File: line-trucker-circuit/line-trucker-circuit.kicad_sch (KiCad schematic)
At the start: 13 parts, among them Q1 Q_Photo_NPN, Q2 Q_Photo_NPN, Q3 Q_Photo_NPN

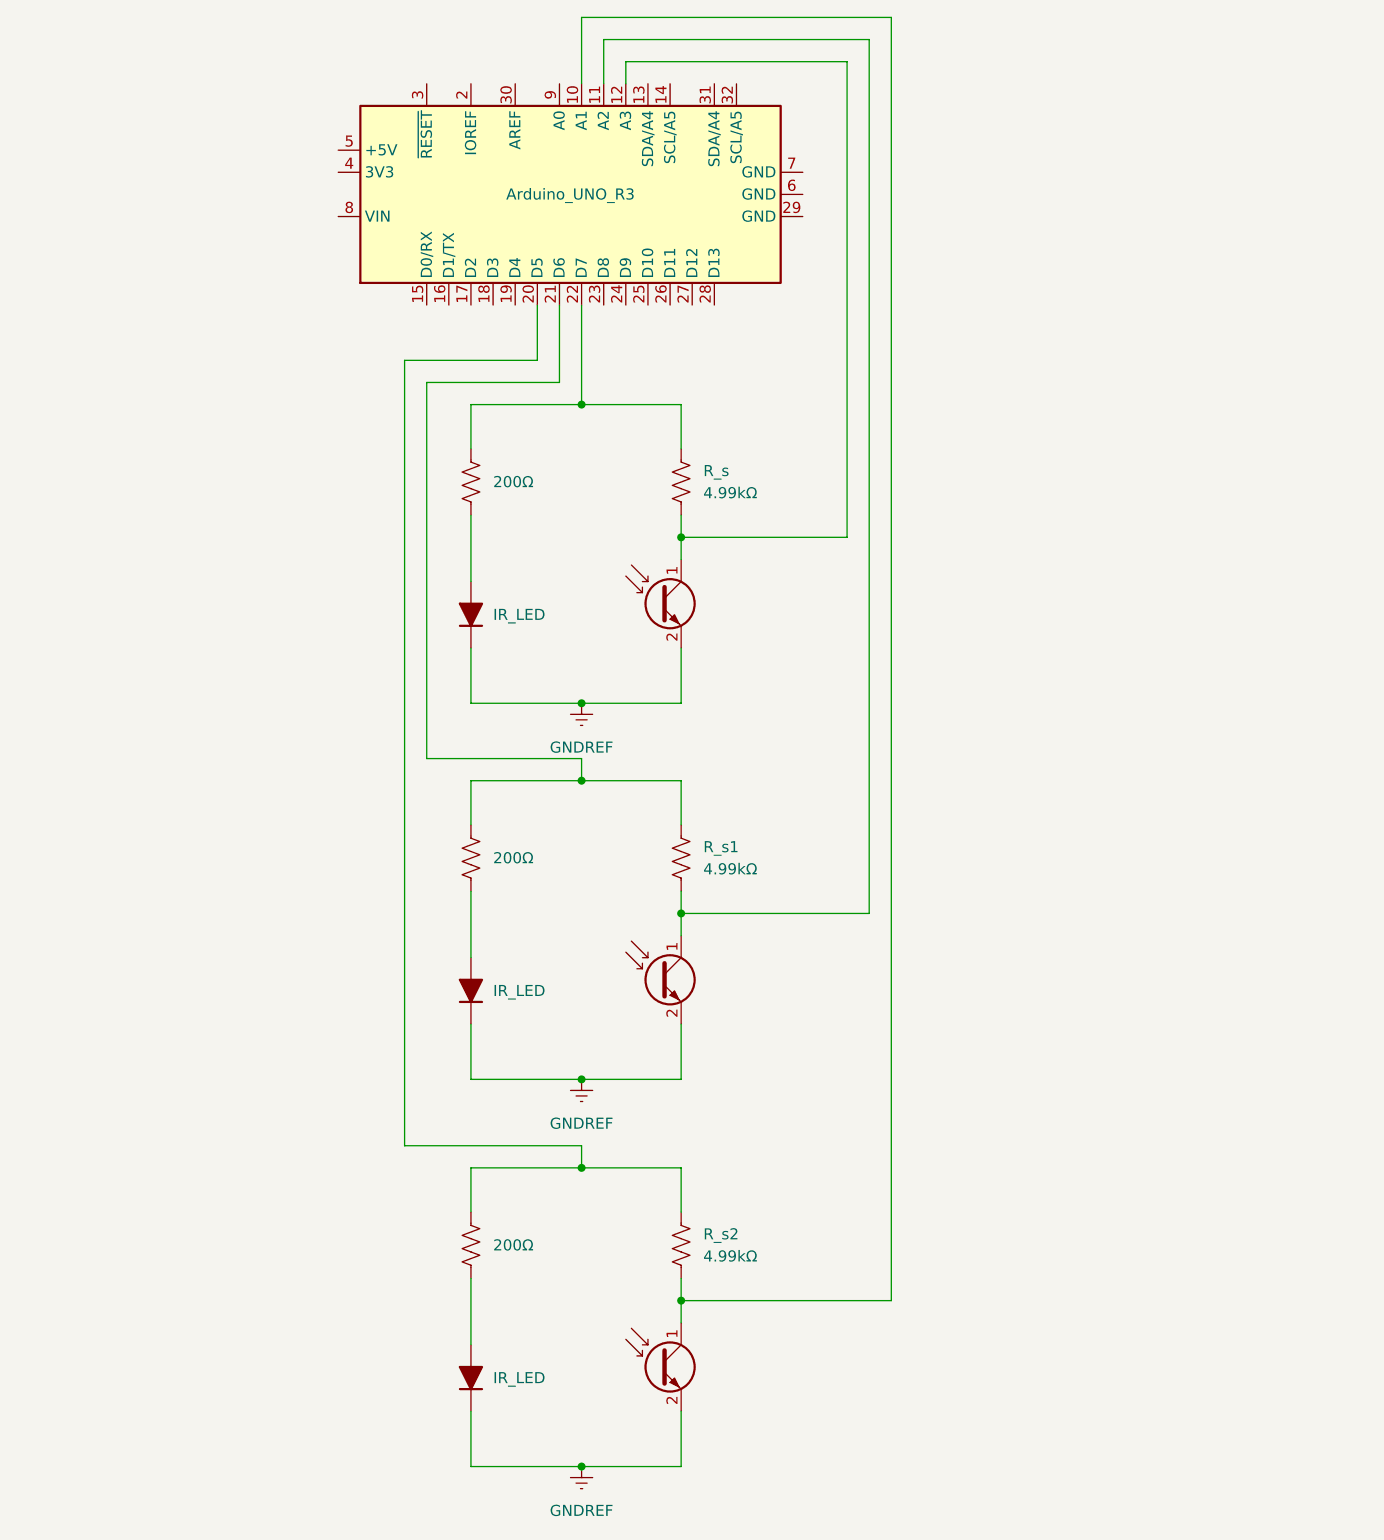
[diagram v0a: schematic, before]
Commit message: Update schematic KiCad file
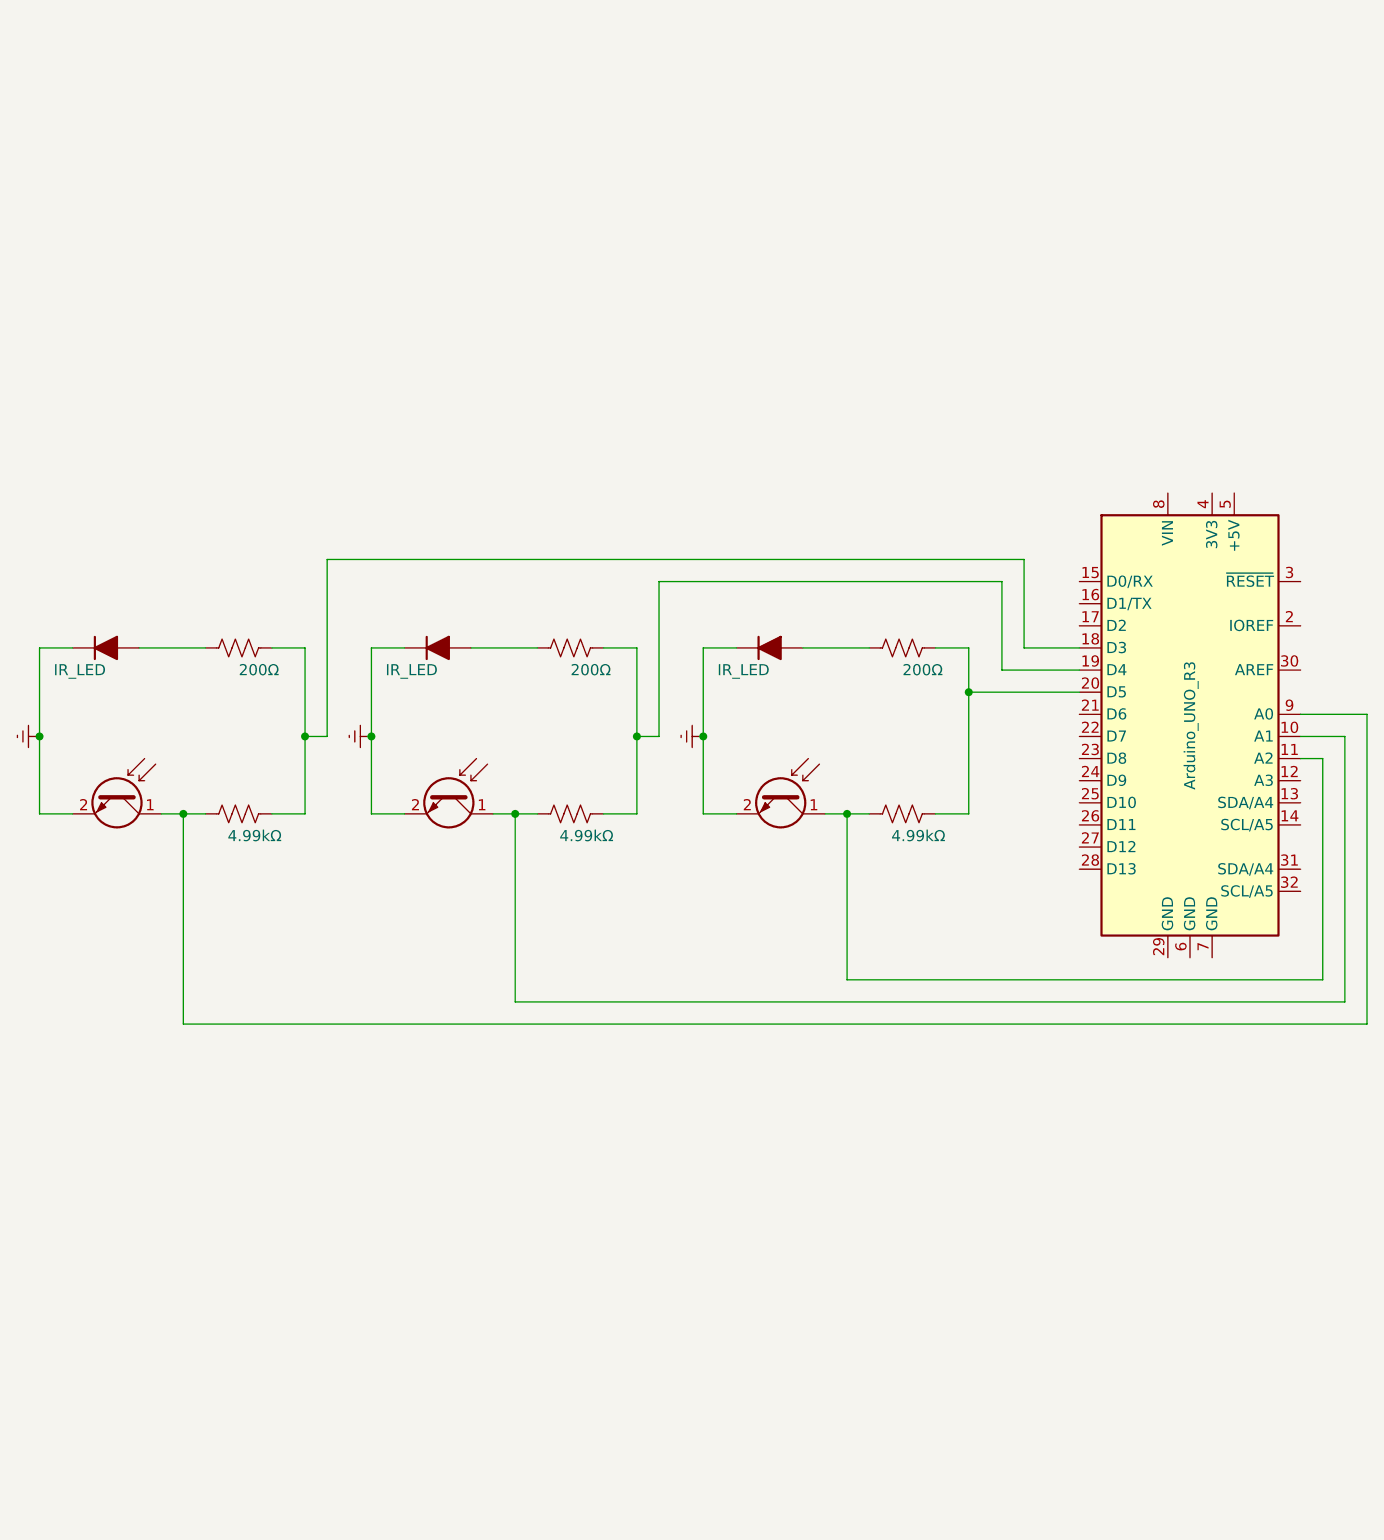
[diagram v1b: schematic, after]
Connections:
- net at R3.1, R_s2.1: now also A1.18 (D3); no longer A1.20 (D5)
- net at Q3.1 (C), R_s2.2: now also A1.9 (A0); no longer A1.10 (A1)
- net at R2.1, R_s1.1: now also A1.19 (D4); no longer A1.21 (D6)
- net at Q2.1 (C), R_s1.2: now also A1.10 (A1); no longer A1.11 (A2)
- net at Q1.1 (C), R_s.2: now also A1.11 (A2); no longer A1.12 (A3)
- net at R1.1, R_s.1: now also A1.20 (D5); no longer A1.22 (D7)
